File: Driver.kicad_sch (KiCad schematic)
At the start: 32 parts

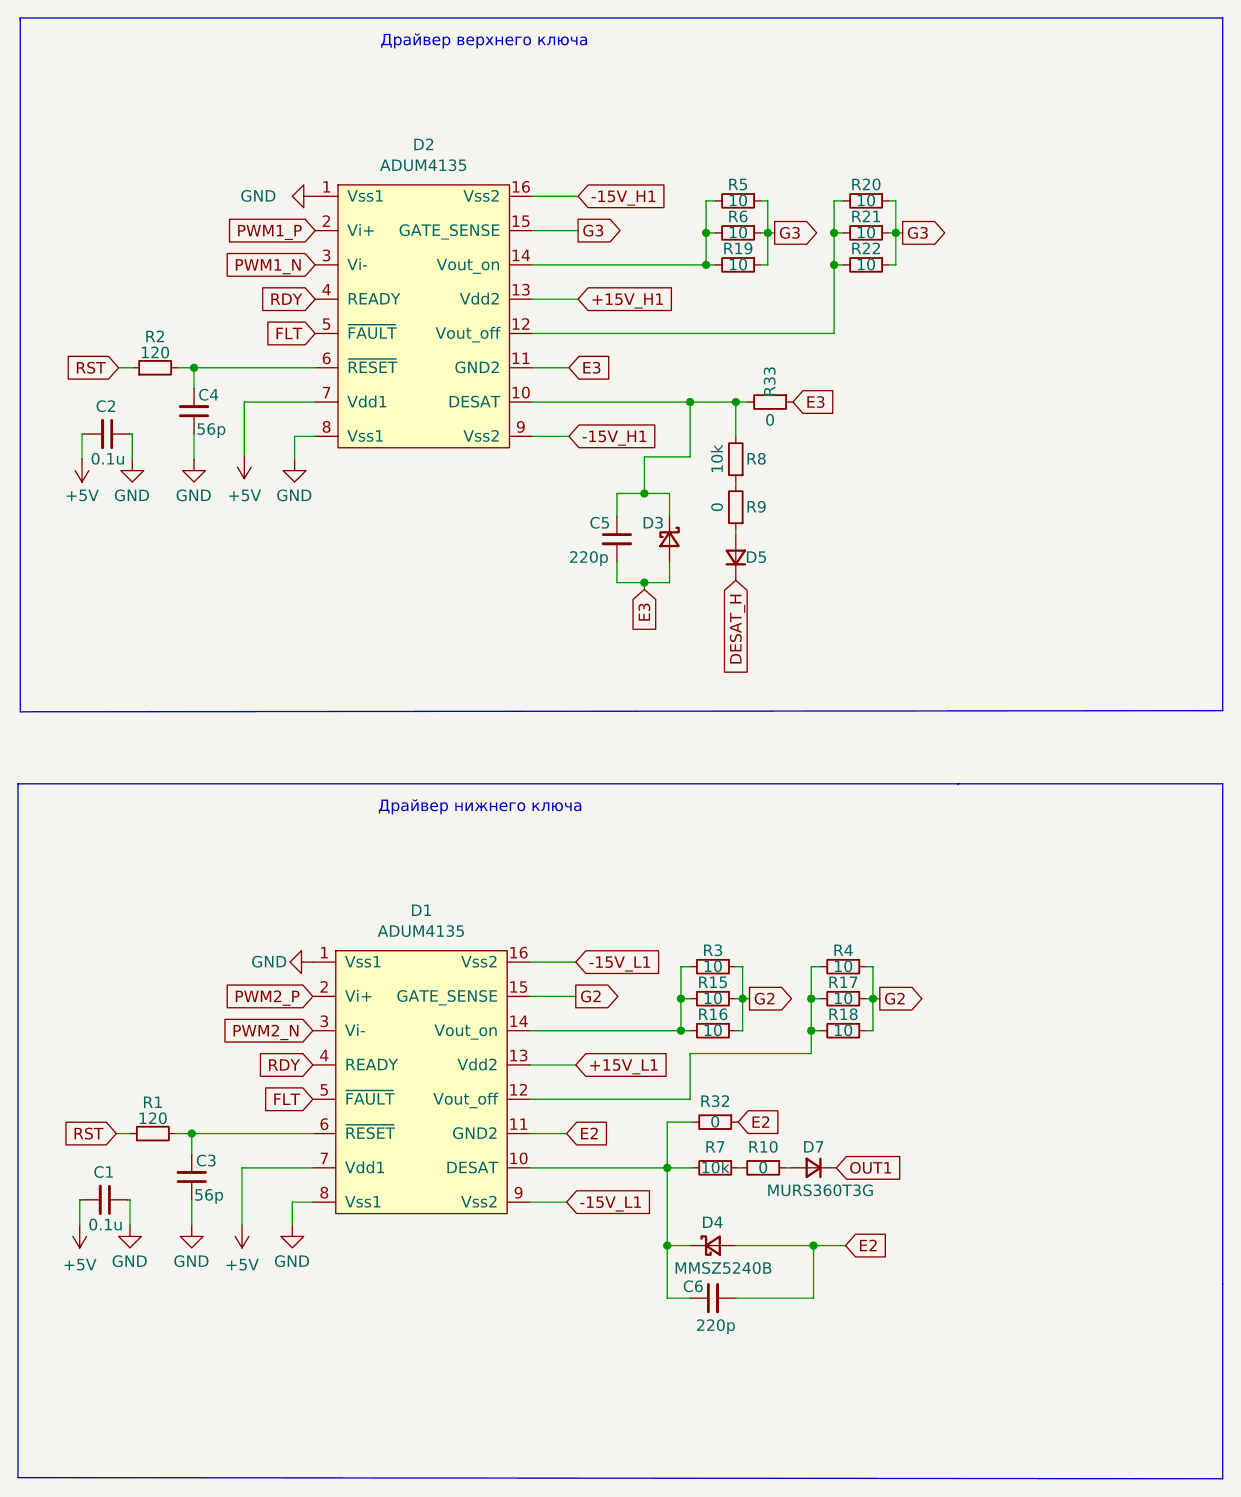
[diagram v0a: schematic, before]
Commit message: Развел все дорожки
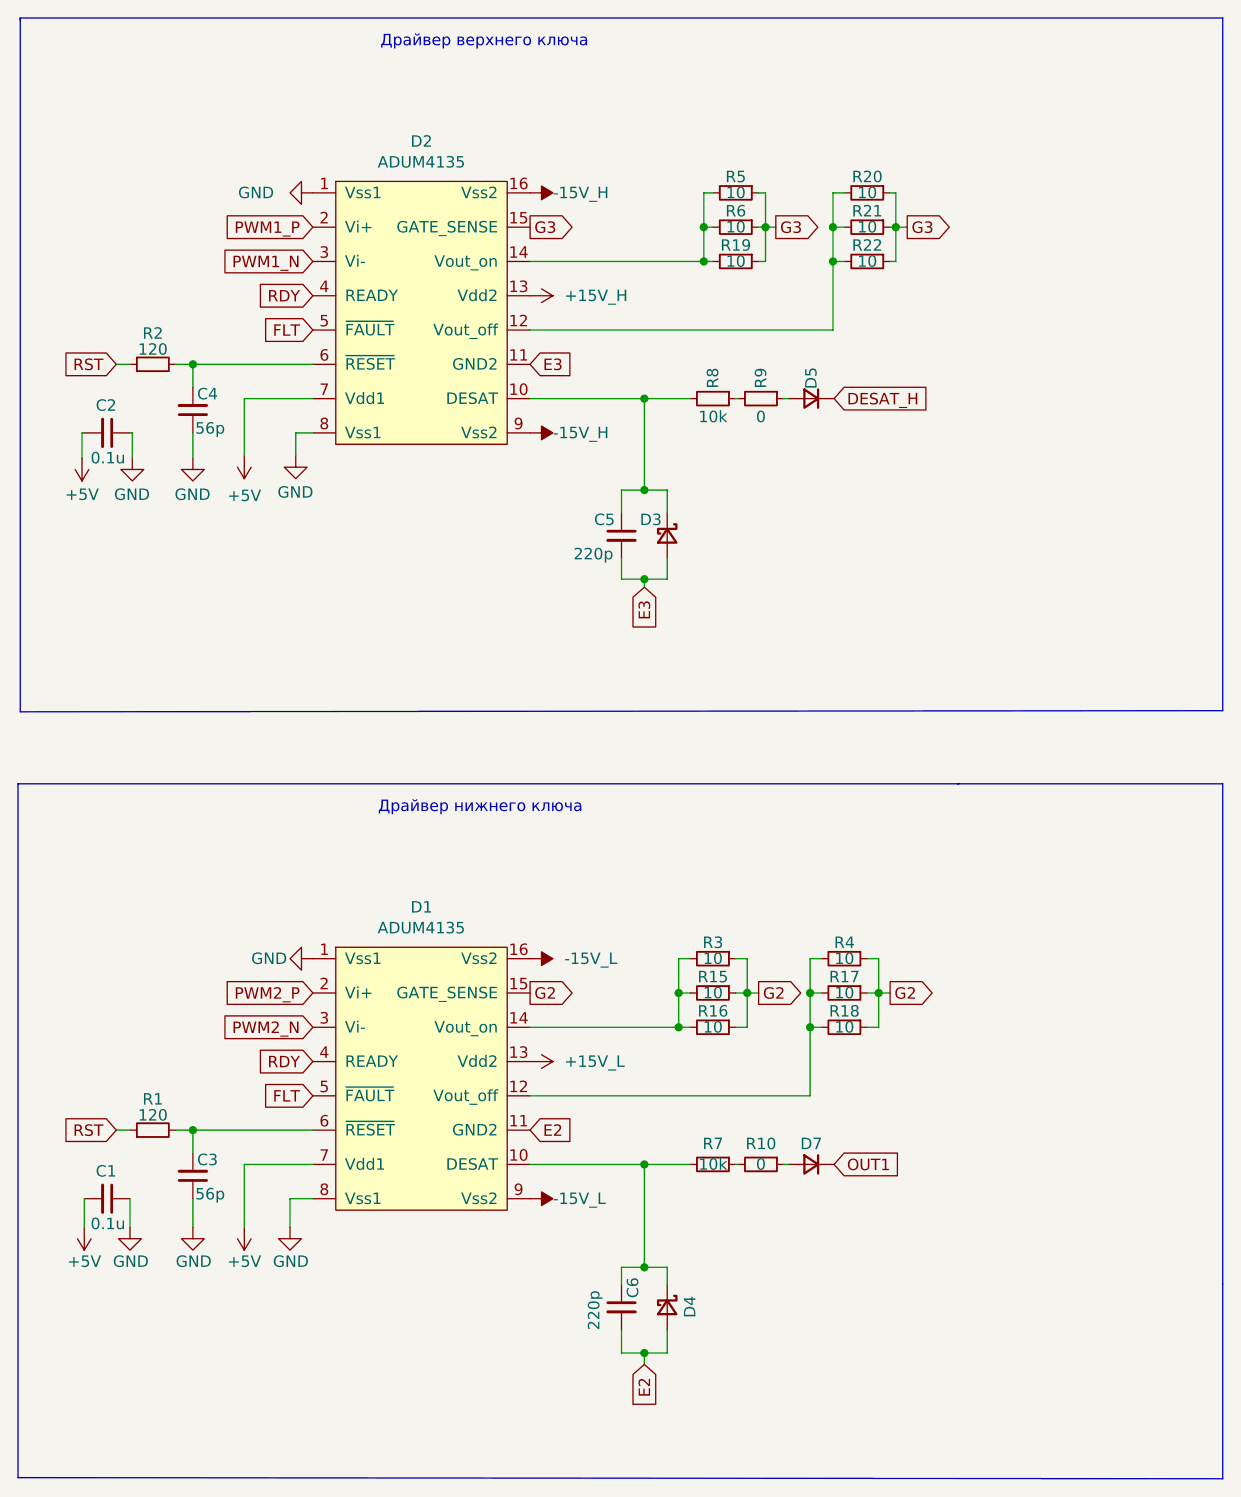
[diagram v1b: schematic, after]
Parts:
- removed R32, R33: 0, Resistor_SMD:R_0805_2012Metric_Pad1.20x1.40mm_HandSolder, symbol Device:R_Small
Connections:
- net +15V_H1 renamed +15V_H
- net +15V_L1 renamed +15V_L
- net -15V_H1 renamed -15V_H
- net -15V_L1 renamed -15V_L
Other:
- moved on the sheet: C5, C6, D4, D5, R15, R17, R20, R21, R3, R4, R5, R6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

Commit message: VER2.0 Отправил в резонит
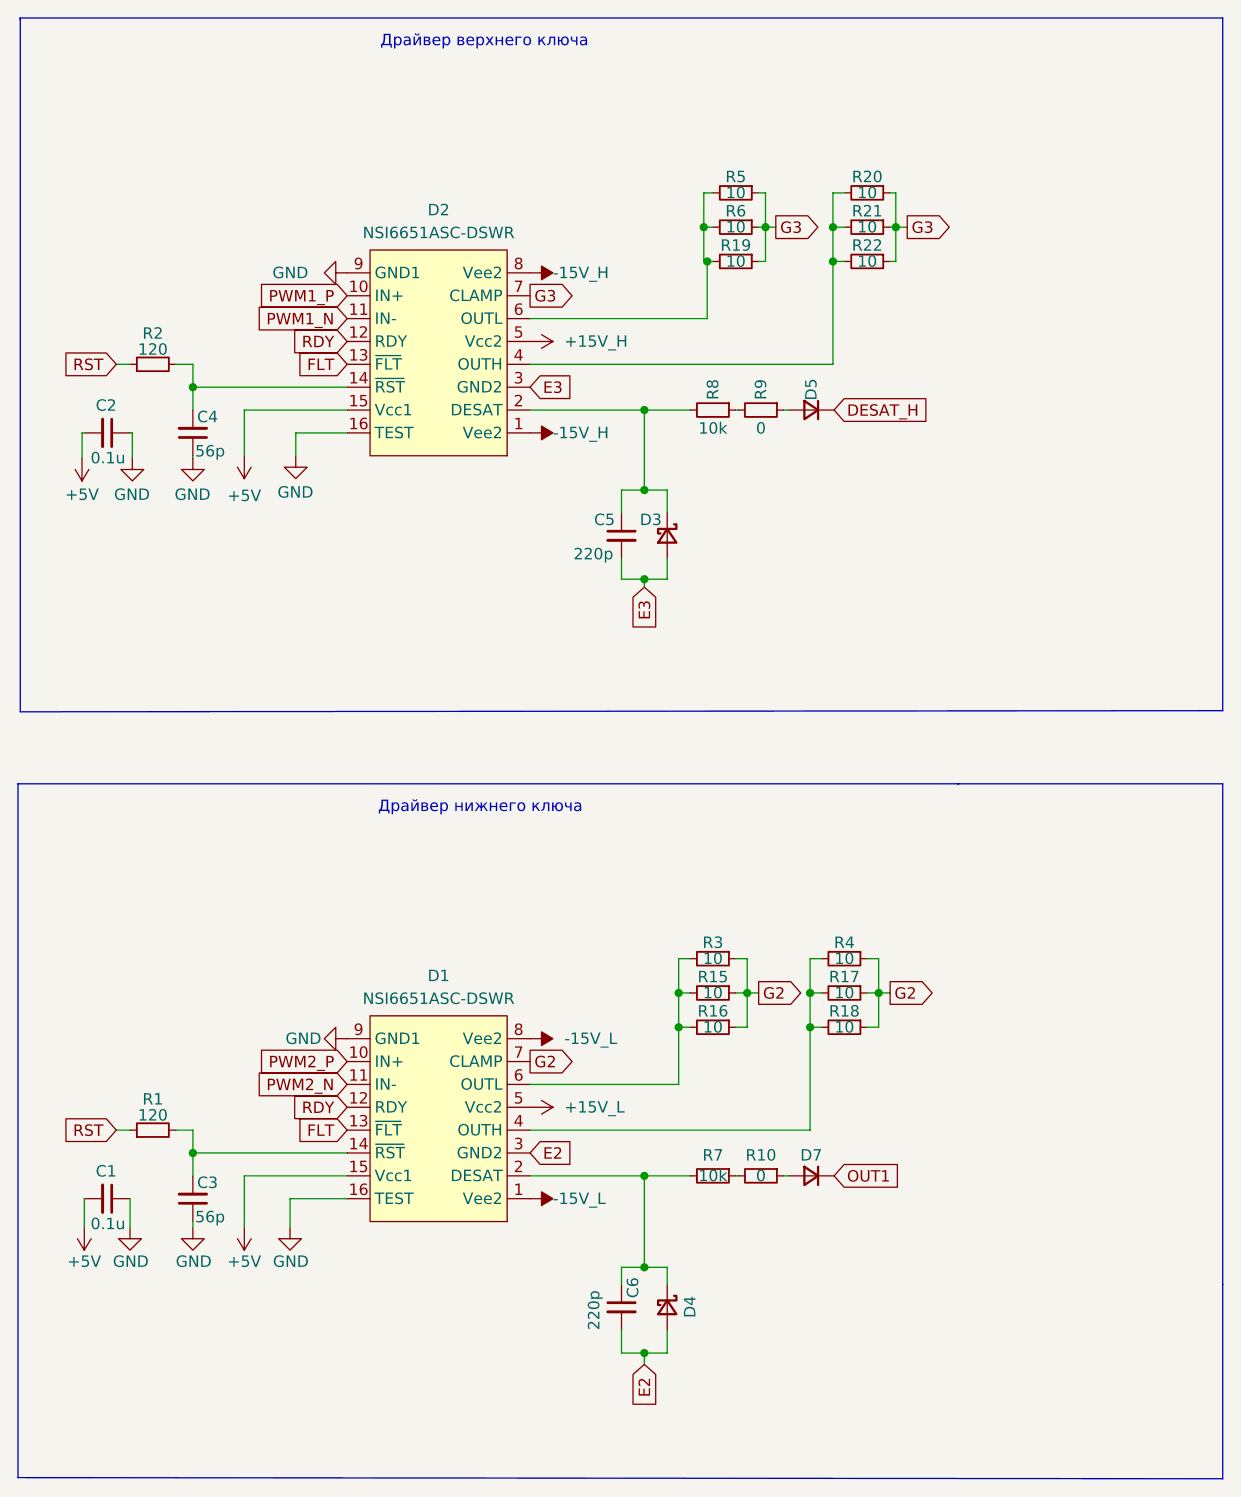
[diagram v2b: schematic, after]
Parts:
- removed D1, D2: ADUM4135, Package_SO:SOIC-16W_7.5x10.3mm_P1.27mm, symbol ADUM_Driver:ADUM4135
- added D1, D2: NSI6651ASC-DSWR, Package_SO:SOIC-16W_7.5x10.3mm_P1.27mm, symbol Driver_My:NSI6651
- D5, D7: value MURS360T3G -> MURS160
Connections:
- net +15V_H: now also D2.5 (Vcc2)
- net +15V_L: now also D1.5 (Vcc2)
- net +5V: now also D1.15 (Vcc1), D2.15 (Vcc1)
- net -15V_H: now also D2.1 (Vee2), D2.8 (Vee2)
- net -15V_L: now also D1.1 (Vee2), D1.8 (Vee2)
- net E2: now also D1.3 (GND2)
- net E3: now also D2.3 (GND2)
- net FLT: now also D1.13 (~{FLT}), D2.13 (~{FLT})
- net G2: now also D1.7 (CLAMP)
- net G3: now also D2.7 (CLAMP)
- net GND: now also D1.16 (TEST), D1.9 (GND1), D2.16 (TEST), D2.9 (GND1)
- net PWM1_N: now also D2.11 (IN-)
- net PWM1_P: now also D2.10 (IN+)
- net PWM2_N: now also D1.11 (IN-)
- net PWM2_P: now also D1.10 (IN+)
- net RDY: now also D1.12 (RDY), D2.12 (RDY)
- net at R20.2, R21.2, R22.2: now also D2.4 (OUTH)
- net at C5.1, D3.1 (K), R8.2: now also D2.2 (DESAT)
- net at R15.2, R16.2, R3.2: now also D1.6 (OUTL)
- net at R19.2, R5.2, R6.2: now also D2.6 (OUTL)
- net at C3.2, R1.2: now also D1.14 (~{RST})
- net at C6.1, D4.1 (K), R7.2: now also D1.2 (DESAT)
- net at C4.2, R2.2: now also D2.14 (~{RST})
- net at R17.2, R18.2, R4.2: now also D1.4 (OUTH)
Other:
- moved on the sheet: C3, C4, D5, D7, R10, R7, R8, R9
